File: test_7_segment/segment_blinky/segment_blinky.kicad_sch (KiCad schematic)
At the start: 6 parts, among them J1 Conn_01x04_Male

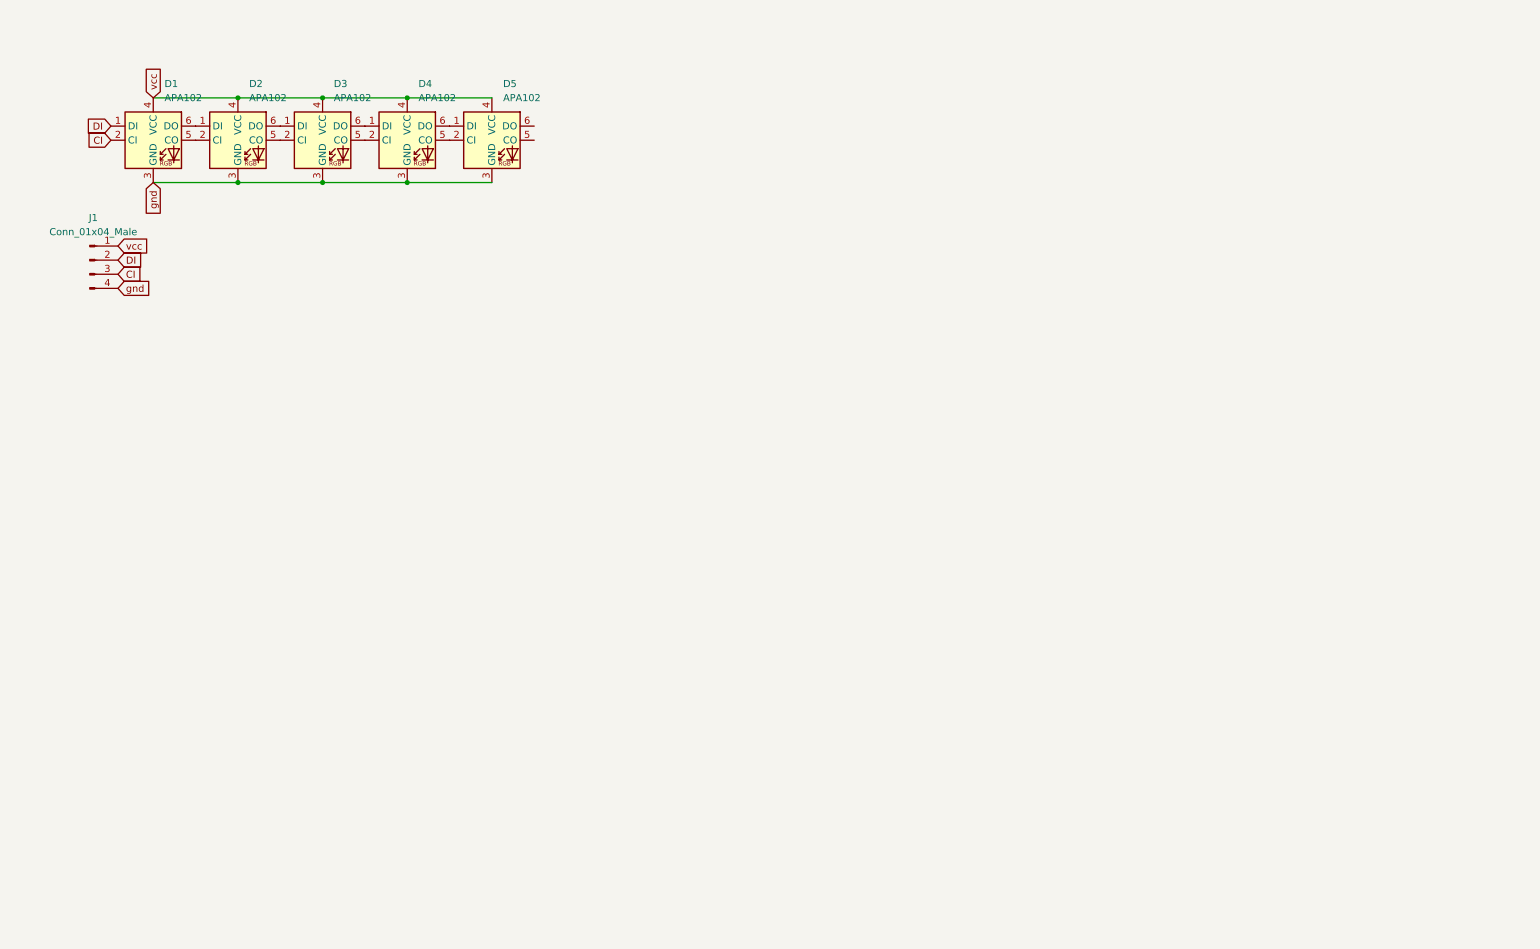
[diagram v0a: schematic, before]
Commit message: Add all the tings for the blinky tests & order it!!
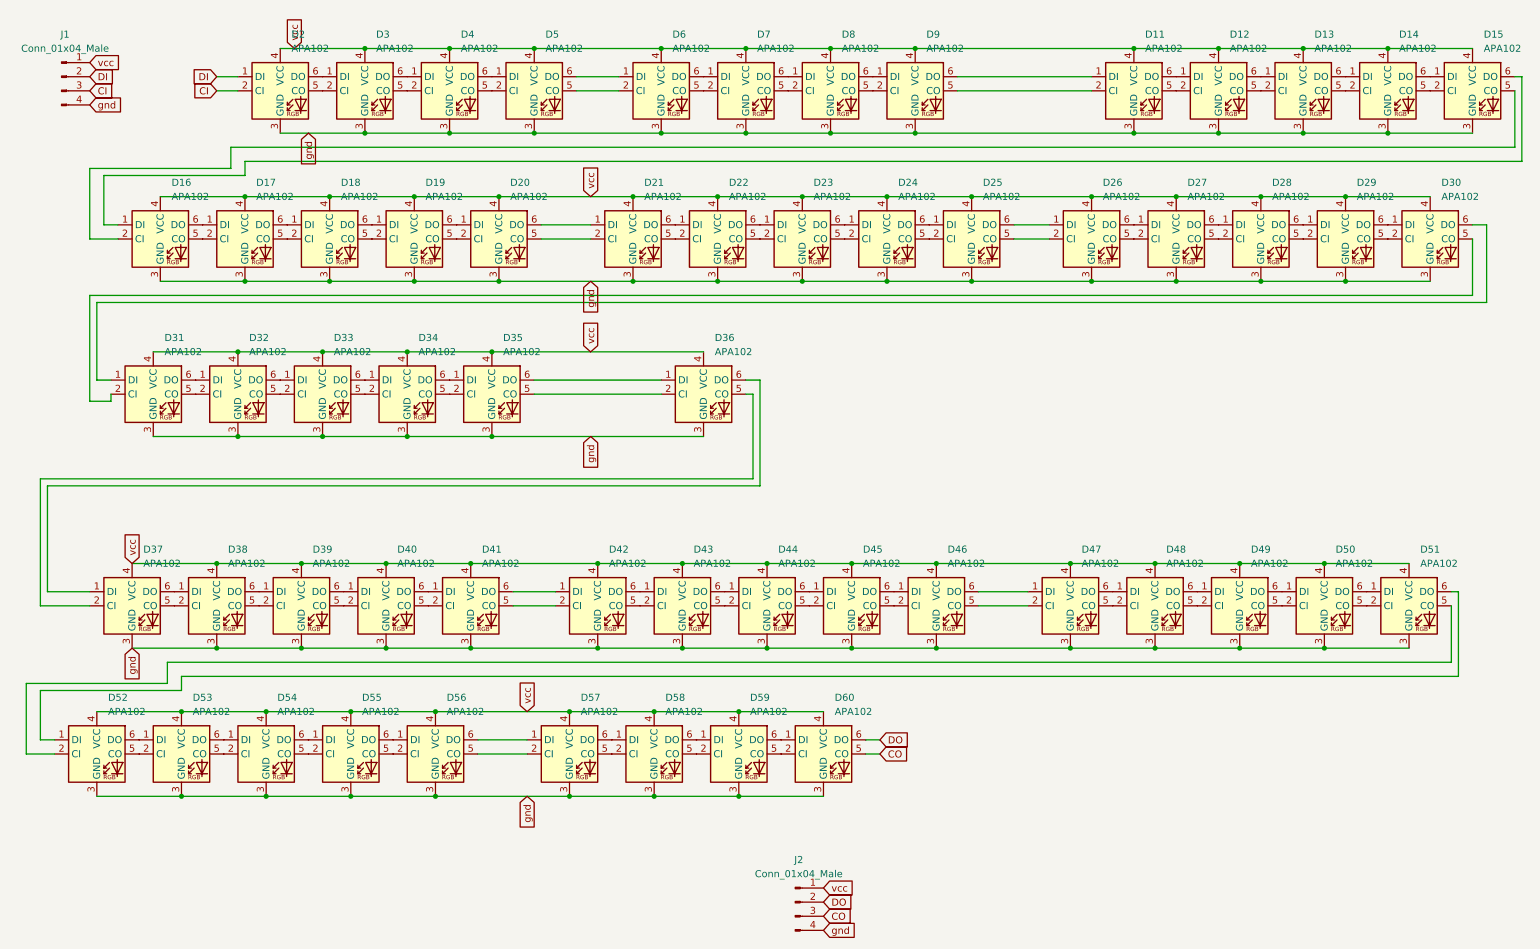
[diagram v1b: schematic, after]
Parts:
- removed D1: APA102, hakz:SK9822-hakz, symbol LED:APA102
- added D11, D12, D13, D14, D15, D16, D17, D18, D19, D20, D21, D22, D23, D24, D25, D26, D27, D28, D29, D30, D31, D32, D33, D34, D35, D36, D37, D38, D39, D40, D41, D42, D43, D44, D45, D46, D47, D48, D49, D50, D51, D52, D53, D54, D55, D56, D57, D58, D59, D6, D60, D7, D8, D9: APA102, hakz:SK9822-hakz, symbol LED:APA102
- added J2: Conn_01x04_Male, Connector_PinHeader_2.54mm:PinHeader_1x04_P2.54mm_Vertical, symbol Connector:Conn_01x04_Male
- J1: footprint (none) -> Connector_PinHeader_2.54mm:PinHeader_1x04_P2.54mm_Vertical
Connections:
- net CI: now also D2.2 (CI)
- net DI: now also D2.1 (DI)
- net gnd: now also D11.3 (GND), D12.3 (GND), D13.3 (GND), D14.3 (GND), D15.3 (GND), D16.3 (GND), D17.3 (GND), D18.3 (GND), D19.3 (GND), D20.3 (GND), D21.3 (GND), D22.3 (GND), D23.3 (GND), D24.3 (GND), D25.3 (GND), D26.3 (GND), D27.3 (GND), D28.3 (GND), D29.3 (GND), D30.3 (GND), D31.3 (GND), D32.3 (GND), D33.3 (GND), D34.3 (GND), D35.3 (GND), D36.3 (GND), D37.3 (GND), D38.3 (GND), D39.3 (GND), D40.3 (GND), D41.3 (GND), D42.3 (GND), D43.3 (GND), D44.3 (GND), D45.3 (GND), D46.3 (GND), D47.3 (GND), D48.3 (GND), D49.3 (GND), D50.3 (GND), D51.3 (GND), D52.3 (GND), D53.3 (GND), D54.3 (GND), D55.3 (GND), D56.3 (GND), D57.3 (GND), D58.3 (GND), D59.3 (GND), D6.3 (GND), D60.3 (GND), D7.3 (GND), D8.3 (GND), D9.3 (GND), J2.4 (Pin_4)
- net vcc: now also D11.4 (VCC), D12.4 (VCC), D13.4 (VCC), D14.4 (VCC), D15.4 (VCC), D16.4 (VCC), D17.4 (VCC), D18.4 (VCC), D19.4 (VCC), D20.4 (VCC), D21.4 (VCC), D22.4 (VCC), D23.4 (VCC), D24.4 (VCC), D25.4 (VCC), D26.4 (VCC), D27.4 (VCC), D28.4 (VCC), D29.4 (VCC), D30.4 (VCC), D31.4 (VCC), D32.4 (VCC), D33.4 (VCC), D34.4 (VCC), D35.4 (VCC), D36.4 (VCC), D37.4 (VCC), D38.4 (VCC), D39.4 (VCC), D40.4 (VCC), D41.4 (VCC), D42.4 (VCC), D43.4 (VCC), D44.4 (VCC), D45.4 (VCC), D46.4 (VCC), D47.4 (VCC), D48.4 (VCC), D49.4 (VCC), D50.4 (VCC), D51.4 (VCC), D52.4 (VCC), D53.4 (VCC), D54.4 (VCC), D55.4 (VCC), D56.4 (VCC), D57.4 (VCC), D58.4 (VCC), D59.4 (VCC), D6.4 (VCC), D60.4 (VCC), D7.4 (VCC), D8.4 (VCC), D9.4 (VCC), J2.1 (Pin_1)
- net at D5.5 (CO): now also D6.2 (CI)
- net at D5.6 (DO): now also D6.1 (DI)
- new net: D20.6 (DO), D21.1 (DI)
- new net: D20.5 (CO), D21.2 (CI)
- new net: D21.5 (CO), D22.2 (CI)
- new net: D21.6 (DO), D22.1 (DI)
- new net: D16.6 (DO), D17.1 (DI)
- new net: D16.5 (CO), D17.2 (CI)
- new net: D17.5 (CO), D18.2 (CI)
- new net: D17.6 (DO), D18.1 (DI)
- new net: D25.6 (DO), D26.1 (DI)
- new net: D25.5 (CO), D26.2 (CI)
- new net: D26.5 (CO), D27.2 (CI)
- new net: D26.6 (DO), D27.1 (DI)
- new net: D6.5 (CO), D7.2 (CI)
- new net: D6.6 (DO), D7.1 (DI)
- new net: D49.6 (DO), D50.1 (DI)
- new net: D49.5 (CO), D50.2 (CI)
- new net: D50.5 (CO), D51.2 (CI)
- new net: D50.6 (DO), D51.1 (DI)
- new net: D56.6 (DO), D57.1 (DI)
- new net: D56.5 (CO), D57.2 (CI)
- new net: D57.5 (CO), D58.2 (CI)
- new net: D57.6 (DO), D58.1 (DI)
- new net: D46.6 (DO), D47.1 (DI)
- new net: D46.5 (CO), D47.2 (CI)
- new net: D47.5 (CO), D48.2 (CI)
- new net: D47.6 (DO), D48.1 (DI)
- new net: D41.6 (DO), D42.1 (DI)
- new net: D41.5 (CO), D42.2 (CI)
- new net: D42.5 (CO), D43.2 (CI)
- new net: D42.6 (DO), D43.1 (DI)
- new net: D31.6 (DO), D32.1 (DI)
- new net: D31.5 (CO), D32.2 (CI)
- new net: D32.5 (CO), D33.2 (CI)
- new net: D32.6 (DO), D33.1 (DI)
- new net: D55.6 (DO), D56.1 (DI)
- new net: D55.5 (CO), D56.2 (CI)
- new net: D38.6 (DO), D39.1 (DI)
- new net: D38.5 (CO), D39.2 (CI)
- new net: D39.5 (CO), D40.2 (CI)
- new net: D39.6 (DO), D40.1 (DI)
- new net: D29.6 (DO), D30.1 (DI)
- new net: D29.5 (CO), D30.2 (CI)
- new net: D30.5 (CO), D31.2 (CI)
- new net: D30.6 (DO), D31.1 (DI)
- new net: D43.5 (CO), D44.2 (CI)
- new net: D43.6 (DO), D44.1 (DI)
- new net: D33.5 (CO), D34.2 (CI)
- new net: D33.6 (DO), D34.1 (DI)
- new net: D22.6 (DO), D23.1 (DI)
- new net: D22.5 (CO), D23.2 (CI)
- new net: D23.5 (CO), D24.2 (CI)
- new net: D23.6 (DO), D24.1 (DI)
- new net: D24.5 (CO), D25.2 (CI)
- new net: D24.6 (DO), D25.1 (DI)
- new net: D18.6 (DO), D19.1 (DI)
- new net: D18.5 (CO), D19.2 (CI)
- new net: D19.5 (CO), D20.2 (CI)
- new net: D19.6 (DO), D20.1 (DI)
- new net: D51.5 (CO), D52.2 (CI)
- new net: D51.6 (DO), D52.1 (DI)
- new net: D48.6 (DO), D49.1 (DI)
- new net: D48.5 (CO), D49.2 (CI)
- new net: D40.6 (DO), D41.1 (DI)
- new net: D40.5 (CO), D41.2 (CI)
- new net: D35.6 (DO), D36.1 (DI)
- new net: D35.5 (CO), D36.2 (CI)
- new net: D36.5 (CO), D37.2 (CI)
- new net: D36.6 (DO), D37.1 (DI)
- new net: D13.6 (DO), D14.1 (DI)
- new net: D13.5 (CO), D14.2 (CI)
- new net: D14.5 (CO), D15.2 (CI)
- new net: D14.6 (DO), D15.1 (DI)
- new net: D45.6 (DO), D46.1 (DI)
- new net: D45.5 (CO), D46.2 (CI)
- new net: D8.6 (DO), D9.1 (DI)
- new net: D8.5 (CO), D9.2 (CI)
- new net: D11.2 (CI), D9.5 (CO)
- new net: D11.1 (DI), D9.6 (DO)
- new net: D15.5 (CO), D16.2 (CI)
- new net: D15.6 (DO), D16.1 (DI)
- new net: D44.6 (DO), D45.1 (DI)
- new net: D44.5 (CO), D45.2 (CI)
- new net: D34.6 (DO), D35.1 (DI)
- new net: D34.5 (CO), D35.2 (CI)
- new net: D27.6 (DO), D28.1 (DI)
- new net: D27.5 (CO), D28.2 (CI)
- new net: D28.5 (CO), D29.2 (CI)
- new net: D28.6 (DO), D29.1 (DI)
- new net: D37.5 (CO), D38.2 (CI)
- new net: D37.6 (DO), D38.1 (DI)
- new net: D54.6 (DO), D55.1 (DI)
- new net: D54.5 (CO), D55.2 (CI)
- new net: D59.6 (DO), D60.1 (DI)
- new net: D59.5 (CO), D60.2 (CI)
- new net: D58.5 (CO), D59.2 (CI)
- new net: D58.6 (DO), D59.1 (DI)
- new net: D12.6 (DO), D13.1 (DI)
- new net: D12.5 (CO), D13.2 (CI)
- new net: D52.5 (CO), D53.2 (CI)
- new net: D52.6 (DO), D53.1 (DI)
- new net: D53.6 (DO), D54.1 (DI)
- new net: D53.5 (CO), D54.2 (CI)
- new net: D7.5 (CO), D8.2 (CI)
- new net: D7.6 (DO), D8.1 (DI)
- new net: D11.6 (DO), D12.1 (DI)
- new net: D11.5 (CO), D12.2 (CI)
- new net CO: D60.5 (CO), J2.3 (Pin_3)
- new net DO: D60.6 (DO), J2.2 (Pin_2)
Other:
- moved on the sheet: D2, D3, D4, D5, J1
